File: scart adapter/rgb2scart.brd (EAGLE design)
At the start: 67 x 39.4 mm, 10 parts, among them J1 AUDIO_JACK_3.5MM_PTH, X1 SCART-F

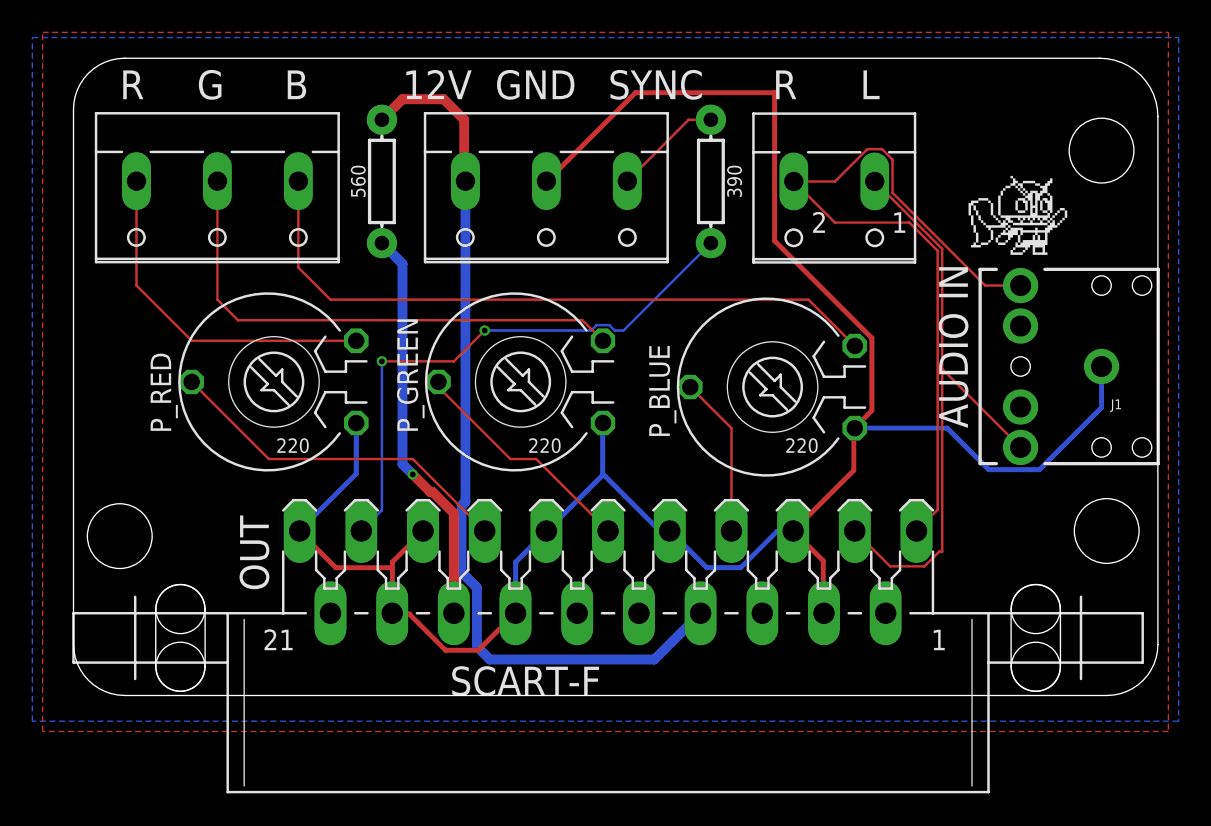
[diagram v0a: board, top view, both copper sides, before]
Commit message: Add files via upload
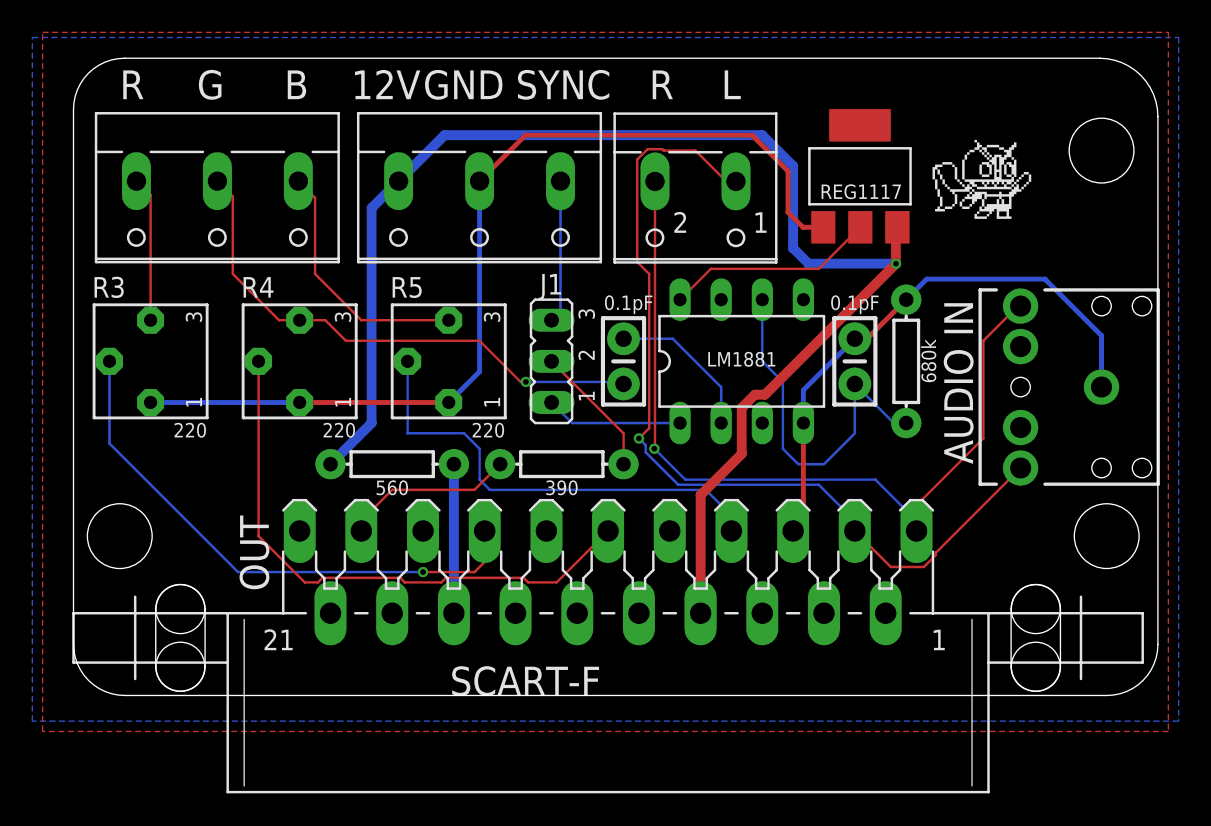
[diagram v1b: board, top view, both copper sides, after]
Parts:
- removed P_BLUE, P_GREEN, P_RED: (no value), pot:PT-10
- added C1, C2: 0.1uF, SparkFun-Capacitors:CAP-PTH-SMALL-KIT
- added IC1: LM1881N, oldchips2:DIL08
- added IC3: REG1117, burr-brown-5:SOT223
- added JP1: (no value), jumper:JP2
- added R3, R4, R5: (no value), bourns:3362P
- added R6: 390, SparkFun-Resistors:AXIAL-0.3
- moved R1 19.7 mm to (30.2, 14.3), turned to 0 degrees
- moved R2 17.5 mm to (19.7, 14.3), turned to 0 degrees
- moved X2 8.57 mm to (38.4, 30.5)
- moved X4 4.13 mm to (25.1, 30.5)
- moved J1 1.27 mm to (63.5, 19.1)
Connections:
- new net 5V: IC1.8, IC3.2
- new net CSYNC: IC1.1, JP1.1
- new net N$1: JP1.2, R1.P$2
- new net N$4: C2.1, IC1.6, R6.P$1
- new net N$5: C1.2, IC1.2
- new net VSYNC: IC1.3
- net 12V: now also IC3.3
- net GND: now also C2.2, IC1.4, IC3.1, R3.1, R4.1, R5.1, R6.P$2; no longer P_BLUE.A, P_GREEN.A, P_RED.A
- net IN_BLUE: now also R5.3; no longer P_BLUE.E
- net IN_GREEN: now also C1.1, R4.3; no longer P_GREEN.E
- net IN_RED: now also R3.3; no longer P_RED.E
- net OUT_BLUE: now also R5.2; no longer P_BLUE.S
- net OUT_GREEN: now also R4.2; no longer P_GREEN.S
- net OUT_RED: now also R3.2; no longer P_RED.S
- net SYNC: now also JP1.3; no longer R1.P$2
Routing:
- net GND: track 133.5 -> 94.0 mm
- net 12V: track 54.5 -> 86.6 mm, vias 0 -> 1
- net IN_BLUE: track 41.7 -> 15.6 mm
- net N$12: track 34.6 -> 10.7 mm, vias 2 -> 0
- net N$4: track 0.00 -> 22.6 mm
- net OUT_GREEN: track 14.5 -> 35.3 mm
- net OUT_BLUE: track 9.94 -> 28.6 mm
- net LEFT: track 38.1 -> 55.1 mm, vias 0 -> 1
- net N$8: track 24.8 -> 9.21 mm, vias 1 -> 0
- net 5V: track 0.00 -> 13.0 mm
- net IN_RED: track 21.4 -> 8.95 mm
- net OUT_RED: track 21.9 -> 33.7 mm, vias 0 -> 1
- net N$5: track 0.00 -> 9.49 mm
- net CSYNC: track 0.00 -> 8.46 mm
- net N$1: track 0.00 -> 8.19 mm
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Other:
- board text added: "0.1pF"
- board text added: "1-2"
- board text added: "2-3"
- board text added: "680k"
- board text added: "J1"
- board text added: "JAMMA"
- board text added: "LM1881"
